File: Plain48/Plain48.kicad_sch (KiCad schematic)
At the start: 0 parts

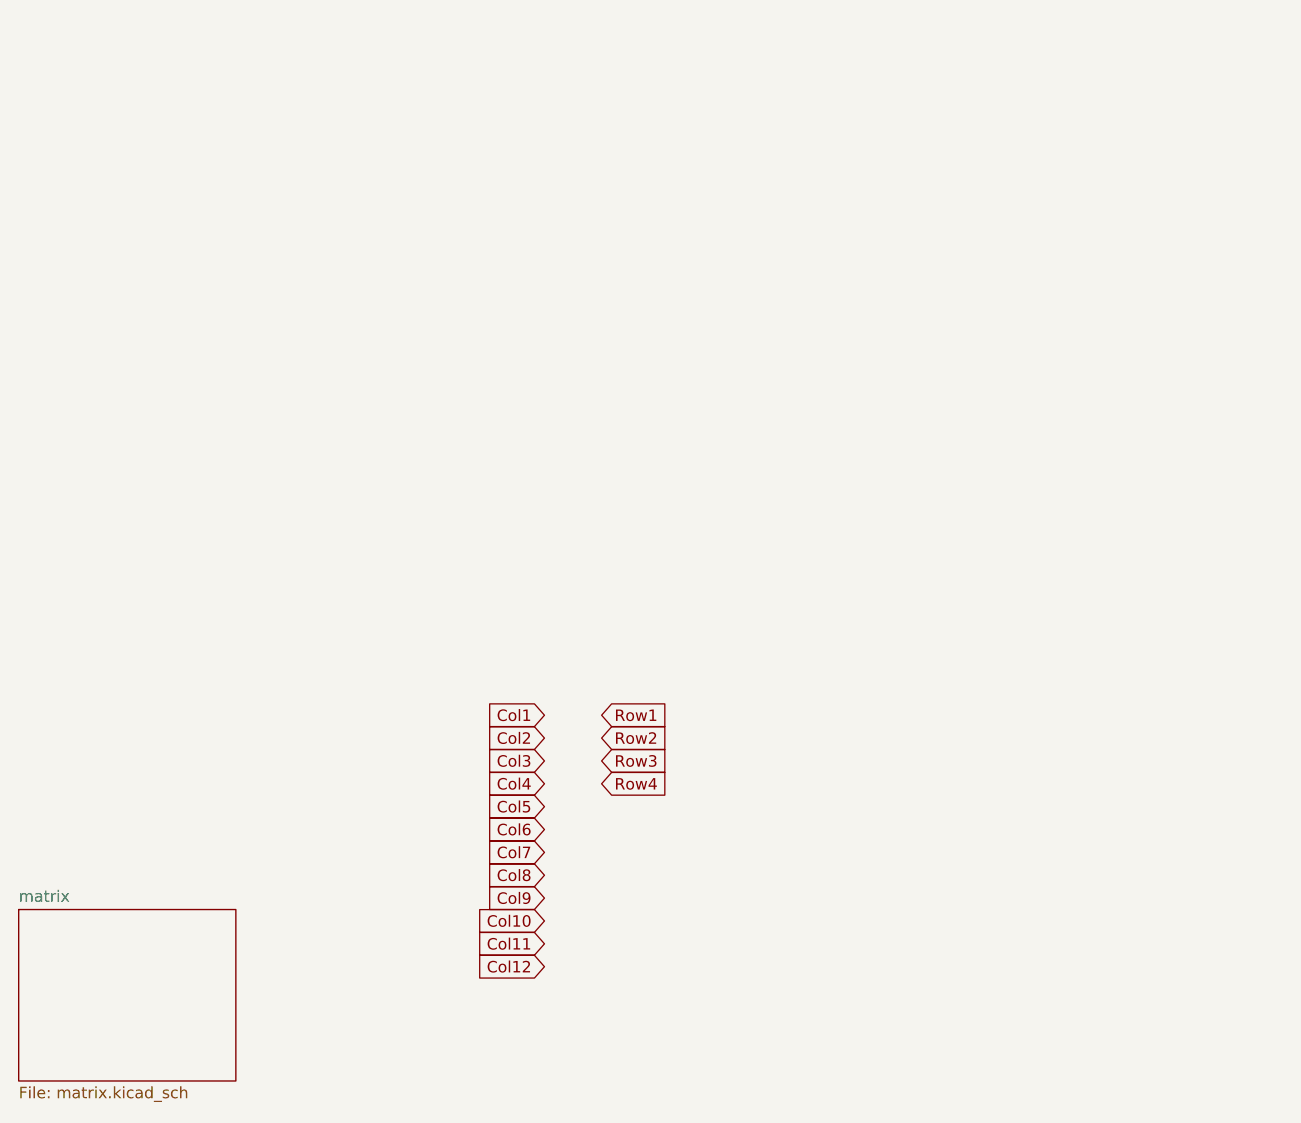
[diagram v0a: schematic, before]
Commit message: upd
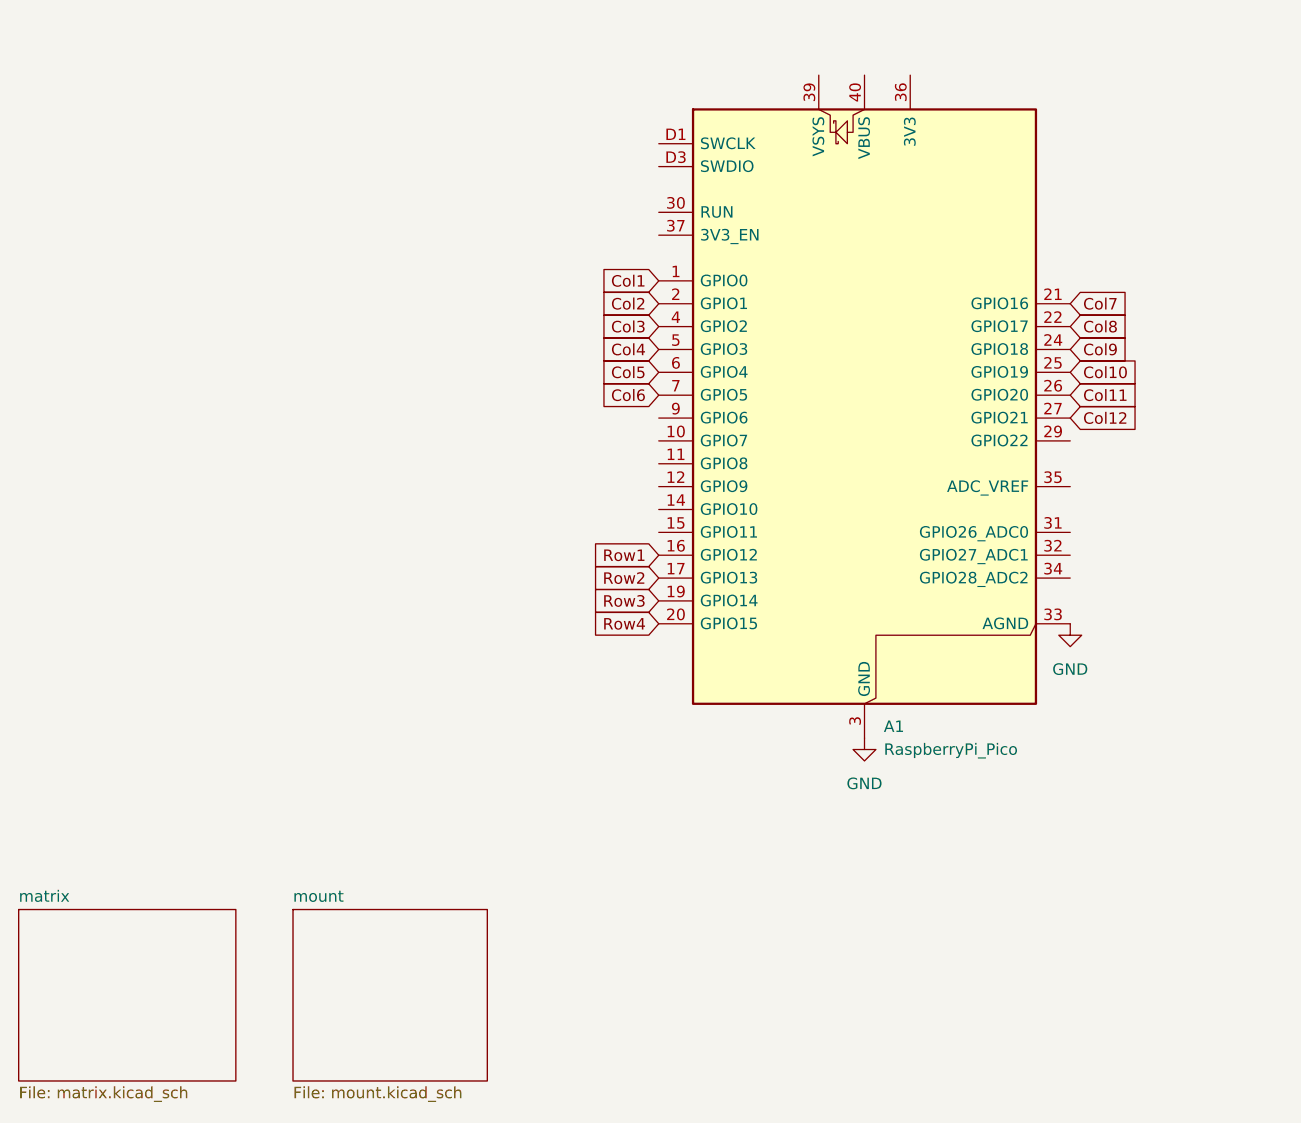
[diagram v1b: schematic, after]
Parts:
- added A1: RaspberryPi_Pico, Module:RaspberryPi_Pico_SMD_HandSolder, symbol MCU_Module:RaspberryPi_Pico_Debug
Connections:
- net Col1: now also A1.1 (GPIO0)
- net Col10: now also A1.25 (GPIO19)
- net Col11: now also A1.26 (GPIO20)
- net Col12: now also A1.27 (GPIO21)
- net Col2: now also A1.2 (GPIO1)
- net Col3: now also A1.4 (GPIO2)
- net Col4: now also A1.5 (GPIO3)
- net Col5: now also A1.6 (GPIO4)
- net Col6: now also A1.7 (GPIO5)
- net Col7: now also A1.21 (GPIO16)
- net Col8: now also A1.22 (GPIO17)
- net Col9: now also A1.24 (GPIO18)
- net Row1: now also A1.16 (GPIO12)
- net Row2: now also A1.17 (GPIO13)
- net Row3: now also A1.19 (GPIO14)
- net Row4: now also A1.20 (GPIO15)
- new net GND: A1.13 (GND), A1.18 (GND), A1.23 (GND), A1.28 (GND), A1.3 (GND), A1.33 (AGND), A1.38 (GND), A1.8 (GND), A1.D2 (GND)
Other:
- added sheet mount (mount.kicad_sch)

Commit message: upd
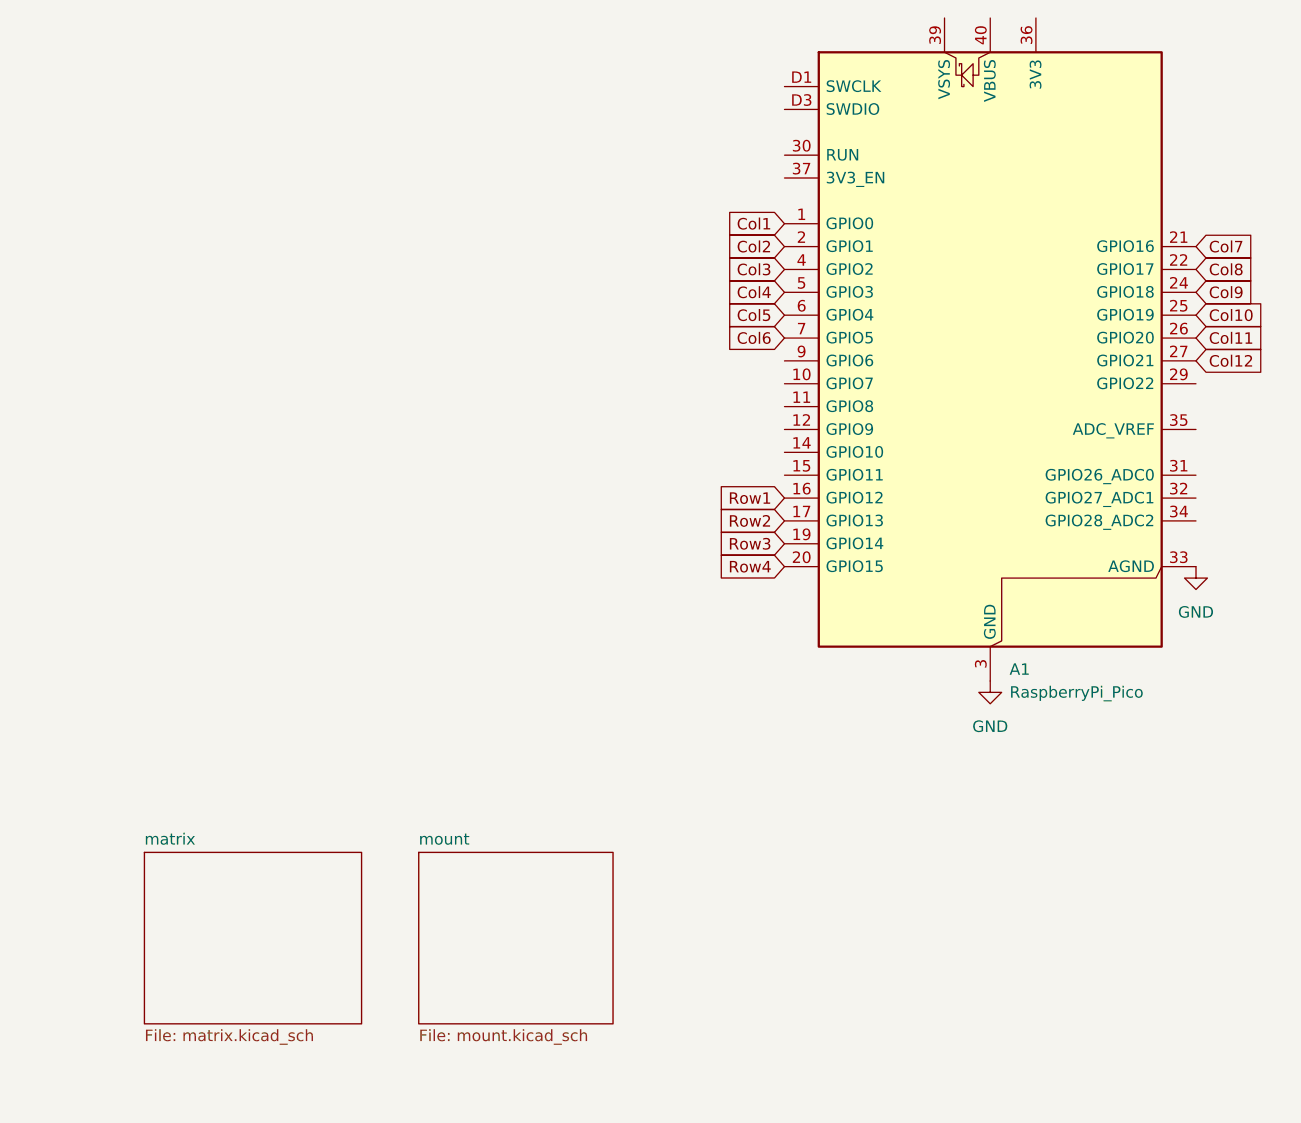
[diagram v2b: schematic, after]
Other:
- company: (none) -> Zero.countersteer
- title: (none) -> Plain 48
- moved on the sheet: A1
